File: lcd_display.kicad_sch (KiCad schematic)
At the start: 1 part, among them P1 OrangePi-2G-IOT LCD Interface

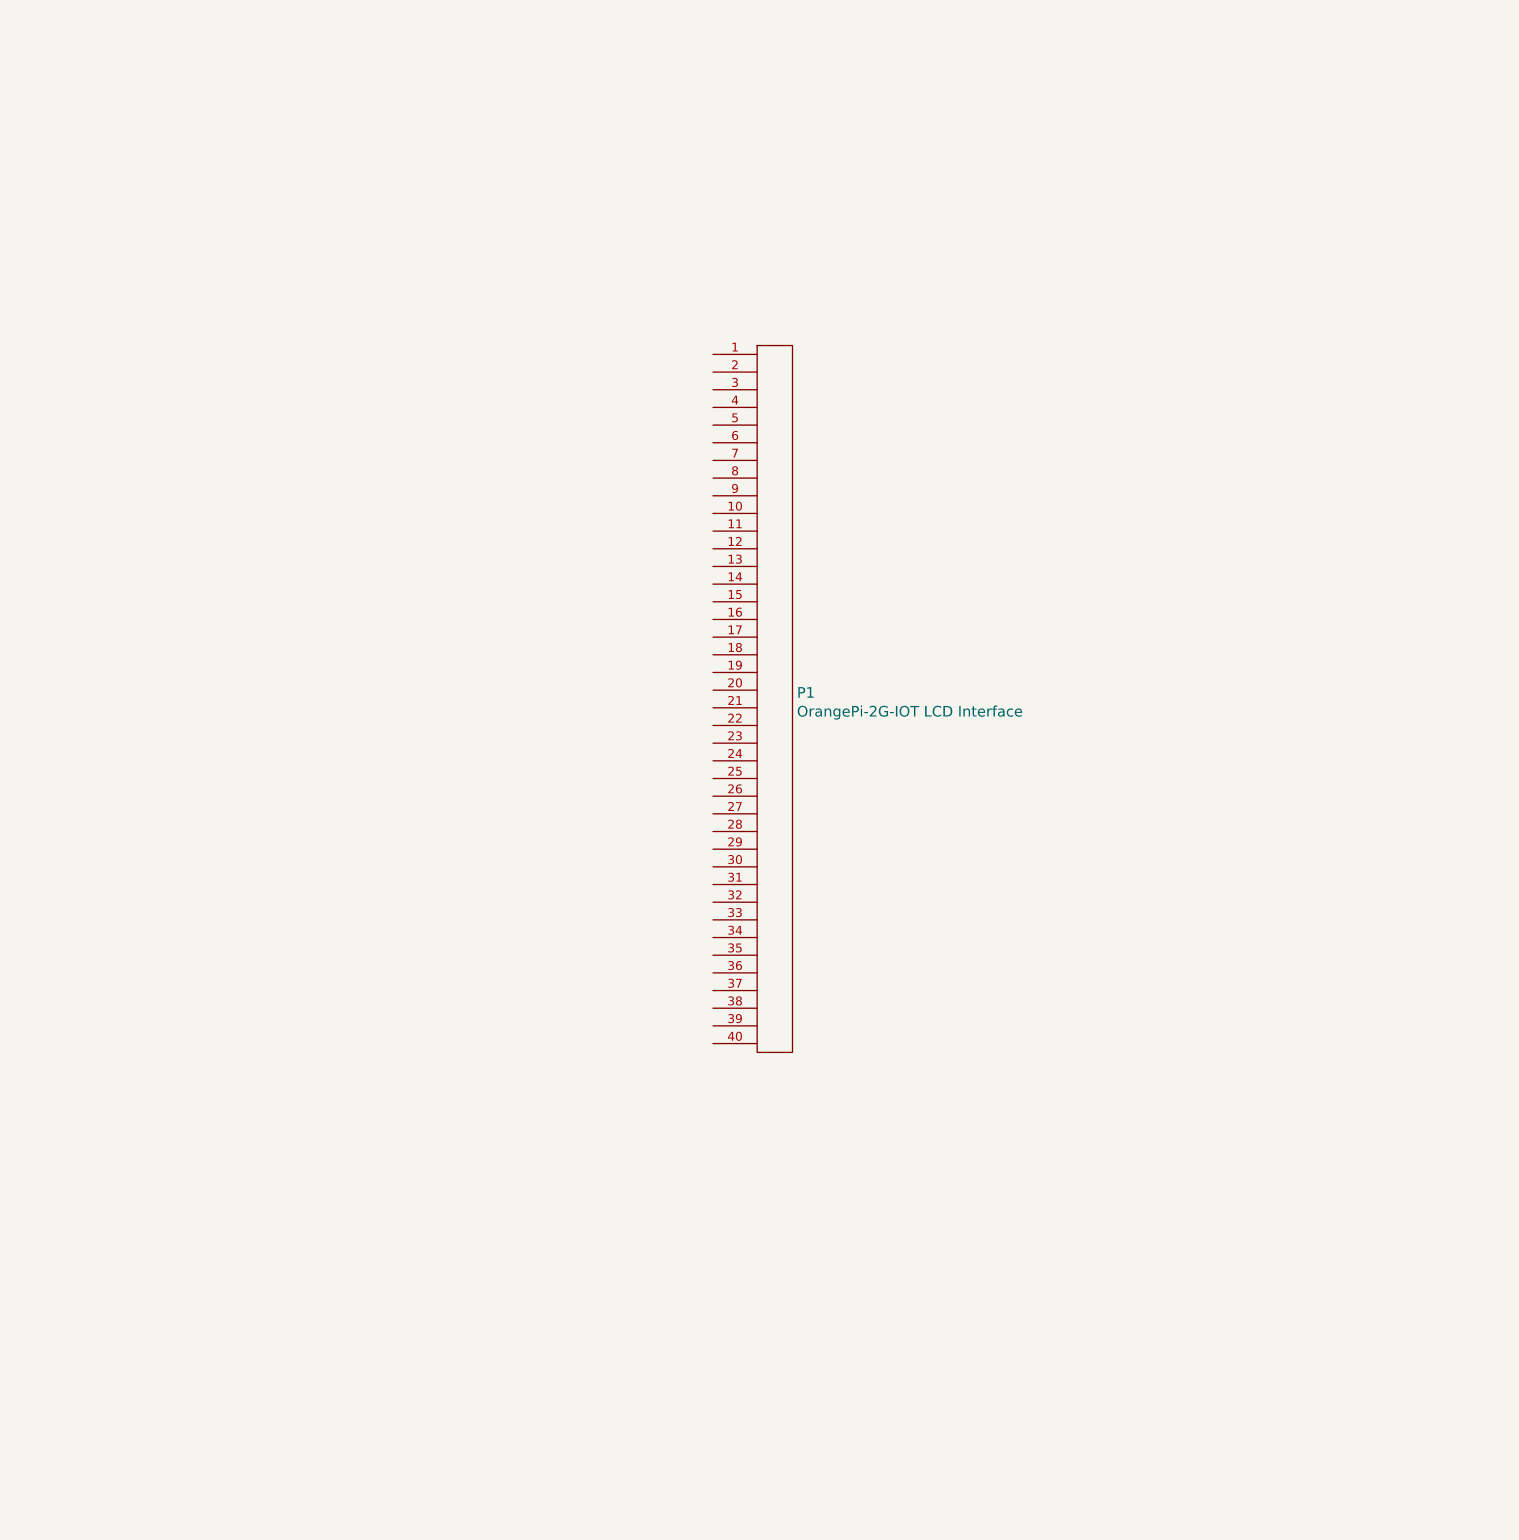
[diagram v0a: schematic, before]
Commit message: Continue schematic work
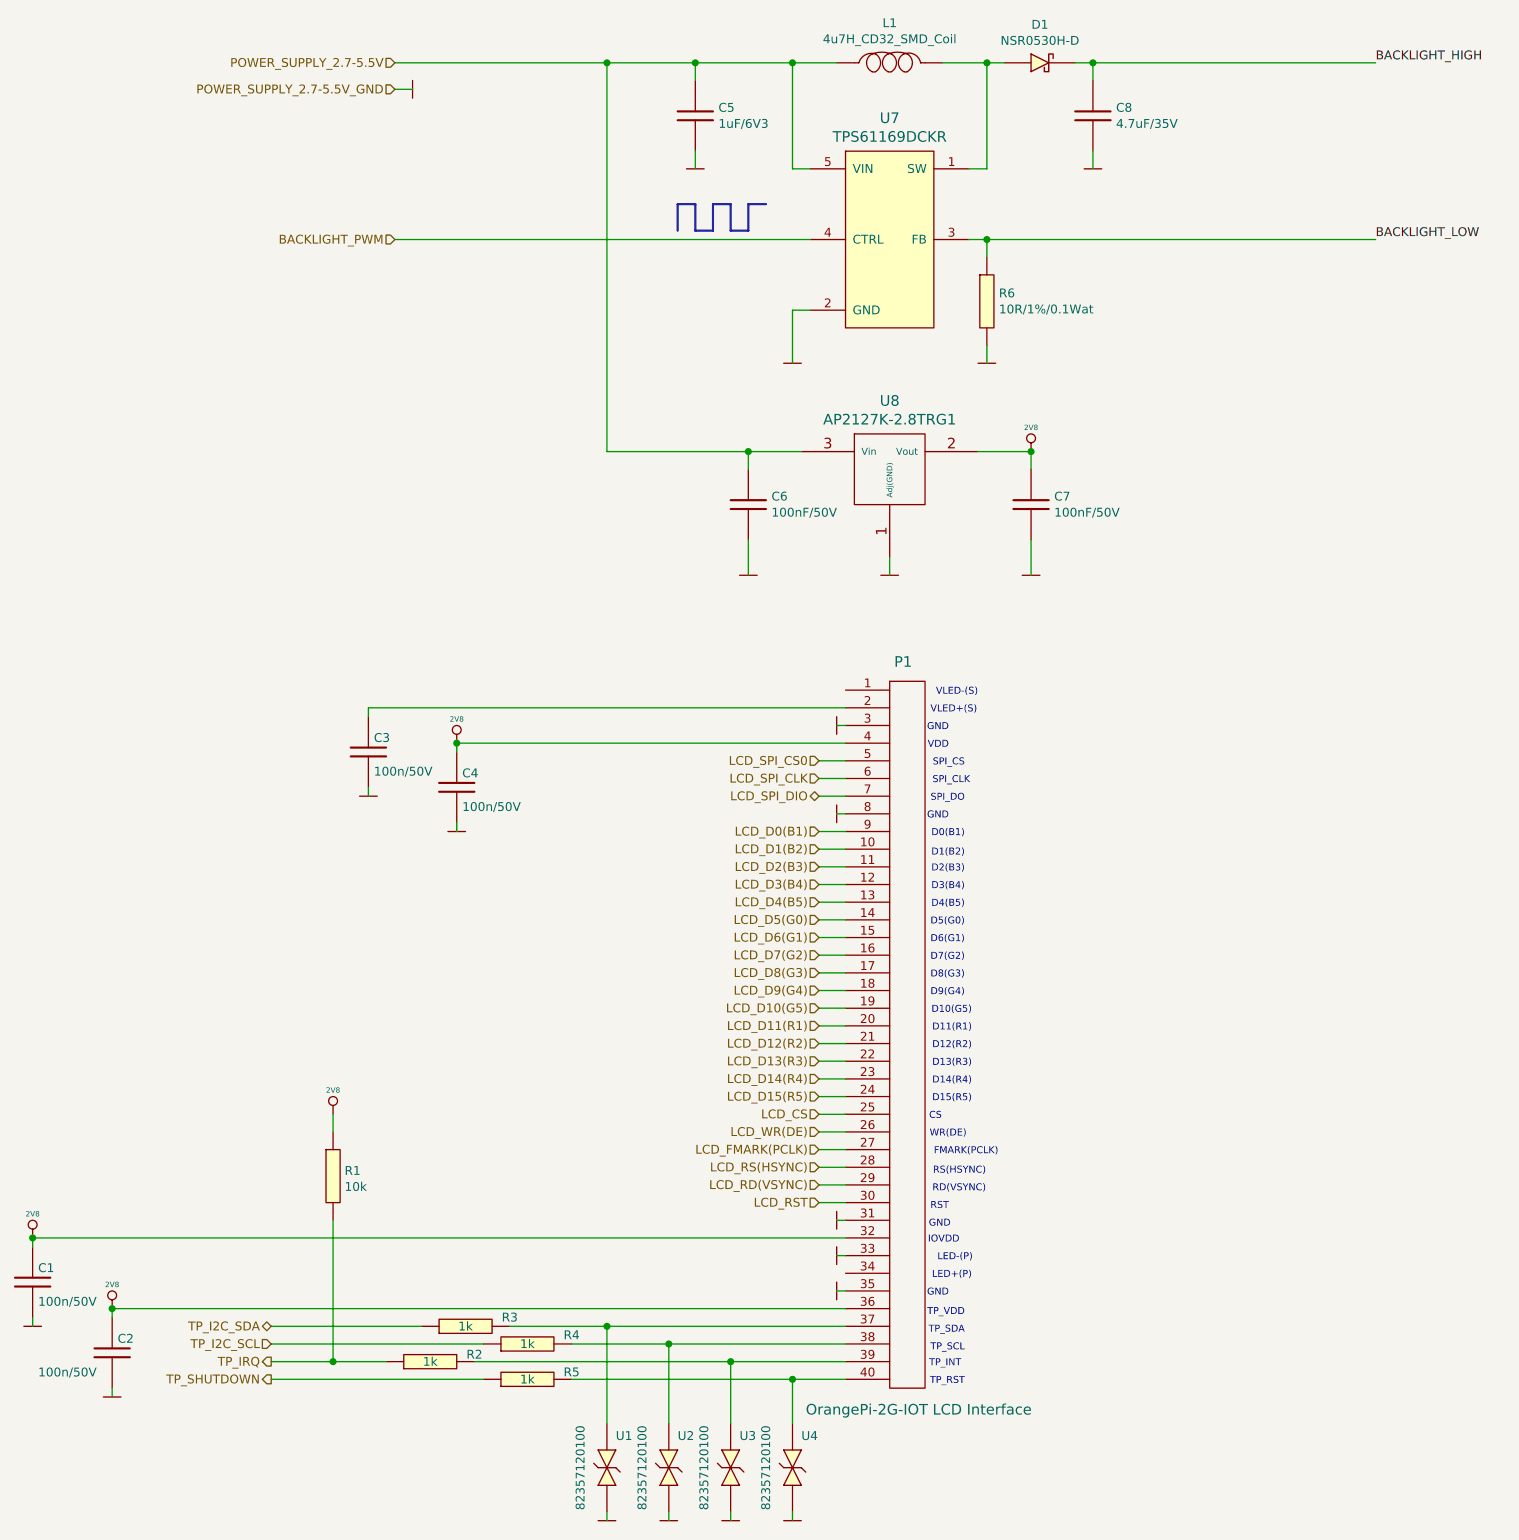
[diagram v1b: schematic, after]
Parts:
- added C1, C2, C3, C4: 100n/50V, Capacitors_Smd_0603:100nF_0603, symbol Capacitors_Smd0603:100n
- added C5: 1uF/6V3, Capacitors_Smd_0603:1uF_0603, symbol Capacitors_Smd0603:1uF_0603
- added C6, C7: 100nF/50V, Capacitors_Smd_0603:100nF_0603, symbol Capacitors_Smd0603:100n
- added C8: 4.7uF/35V, Capacitors_Smd_0603:4_7uF_0603, symbol Capacitors_Smd0603:4_7uF_0603
- added D1: NSR0530H-D, Diodes:NSR0530H-D_SOD323, symbol Diodes:NSR0530H-D
- added L1: 4u7H_CD32_SMD_Coil, Inductors:4u7H_SMD_CD32, symbol Inductors:4u7H_CD32_SMD_Coil
- added R1: 10k, Resistor_Smd_0603:10k_0603, symbol Resistors_Smd0603:10k
- added R2, R3, R4, R5: 1k, Resistor_Smd_0603:1k_0603, symbol Resistors_Smd0603:1k_0603
- added R6: 10R/1%/0.1Wat, Resistor_Smd_0603:10R_0603, symbol Resistors_Smd0603:10R_1%
- added U1, U2, U3, U4: 82357120100, ESD_Protectors:82357120100, symbol esd_protectors:82357120100
- added U7: TPS61169DCKR, Lcd_Backlight_Drivers:TPS61169DCKR, symbol Lcd_Backlight_Drivers:TPS61169DCKR
- added U8: AP2127K-2.8TRG1, Linear:AP2127K-2.8TRG1_SOT23, symbol Linear_Regulators:AP2127K-2.8TRG1
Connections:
- net LCD_D1(B2): now reaches P1.10 (P10)
- net LCD_D2(B3): now reaches P1.11 (P1)
- net LCD_D3(B4): now reaches P1.12 (P2)
- net LCD_D4(B5): now reaches P1.13 (P3)
- net LCD_D5(G0): now reaches P1.14 (P4)
- net LCD_D6(G1): now reaches P1.15 (P5)
- net LCD_D7(G2): now reaches P1.16 (P6)
- net LCD_D8(G3): now reaches P1.17 (P7)
- net LCD_D9(G4): now reaches P1.18 (P8)
- net LCD_D10(G5): now reaches P1.19 (P9)
- net at P1.2 (P2): now also C3.1
- net LCD_D11(R1): now reaches P1.20 (P10)
- net LCD_D12(R2): now reaches P1.21 (P1)
- net LCD_D13(R3): now reaches P1.22 (P2)
- net LCD_D14(R4): now reaches P1.23 (P3)
- net LCD_D15(R5): now reaches P1.24 (P4)
- net LCD_CS: now reaches P1.25 (P5)
- net LCD_WR(DE): now reaches P1.26 (P6)
- net LCD_FMARK(PCLK): now reaches P1.27 (P7)
- net LCD_RS(HSYNC): now reaches P1.28 (P8)
- net LCD_RD(VSYNC): now reaches P1.29 (P9)
- net GND: now reaches P1.3 (P3)
- net GND: now also P1.31 (P1), P1.33 (P3), P1.35 (P5), P1.8 (P8), C1.2, C2.2, C3.2, C4.2, C5.2, C6.2, C7.2, C8.2, R6.2, U1.1 (A), U2.1 (A), U3.1 (A), U4.1 (A), U7.2 (GND), U8.1 (Adj(GND))
- net LCD_RST: now reaches P1.30 (P10)
- net 2V8: now reaches P1.32 (P2)
- net 2V8: now also P1.36 (P6), P1.4 (P4), C1.1, C2.1, C4.1, C7.1, R1.1, U8.2 (Vout)
- net at P1.37 (P7): now also R3.2, U1.2 (K)
- net at P1.38 (P8): now also R4.2, U2.2 (K)
- net at P1.39 (P9): now also R2.2, U3.2 (K)
- net at P1.40 (P10): now also R5.2, U4.2 (K)
- net LCD_SPI_CS0: now reaches P1.5 (P5)
- net LCD_SPI_CLK: now reaches P1.6 (P6)
- net LCD_SPI_DIO: now reaches P1.7 (P7)
- net LCD_D0(B1): now reaches P1.9 (P9)
- new net: D1.2 (A), L1.2, U7.1 (SW)
- new net BACKLIGHT_HIGH: C8.1, D1.1 (K)
- new net BACKLIGHT_LOW: R6.1, U7.3 (FB)
- new net BACKLIGHT_PWM: U7.4 (CTRL)
- new net POWER_SUPPLY_2.7-5.5V: C5.1, C6.1, L1.1, U7.5 (VIN), U8.3 (Vin)
- new net TP_I2C_SCL: R4.1
- new net TP_I2C_SDA: R3.1
- new net TP_IRQ: R1.2, R2.1
- new net TP_SHUTDOWN: R5.1
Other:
- note added: "CS"
- note added: "D0(B1)"
- note added: "D1(B2)"
- note added: "D10(G5)"
- note added: "D11(R1)"
- note added: "D12(R2)"
- note added: "D13(R3)"
- note added: "D14(R4)"
- note added: "D15(R5)"
- note added: "D2(B3)"
- note added: "D3(B4)"
- note added: "D4(B5)"
- note added: "D5(G0)"
- note added: "D6(G1)"
- note added: "D7(G2)"
- note added: "D8(G3)"
- note added: "D9(G4)"
- note added: "FMARK(PCLK)"
- note added: "GND"
- note added: "IOVDD"
- note added: "LED+(P)"
- note added: "LED-(P)"
- note added: "RD(VSYNC)"
- note added: "RS(HSYNC)"
- note added: "RST"
- note added: "SPI_CLK"
- note added: "SPI_CS"
- note added: "SPI_DO"
- note added: "TP_INT"
- note added: "TP_RST"
- note added: "TP_SCL"
- note added: "TP_SDA"
- note added: "TP_VDD"
- note added: "VDD"
- note added: "VLED+(S)"
- note added: "VLED-(S)"
- note added: "WR(DE)"
- moved on the sheet: P1
